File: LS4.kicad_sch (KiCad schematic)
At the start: 6 parts, among them U7 VNLD5160TR-E, U8 VNLD5160TR-E

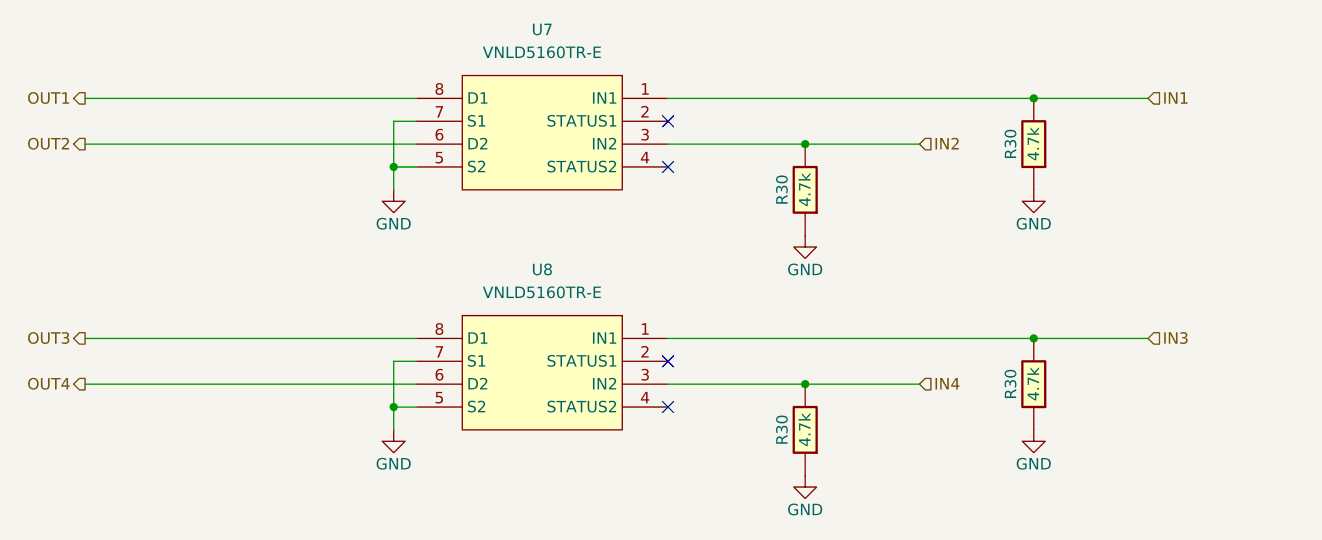
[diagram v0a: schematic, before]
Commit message: Unification with UAEFI F7 #114 #110
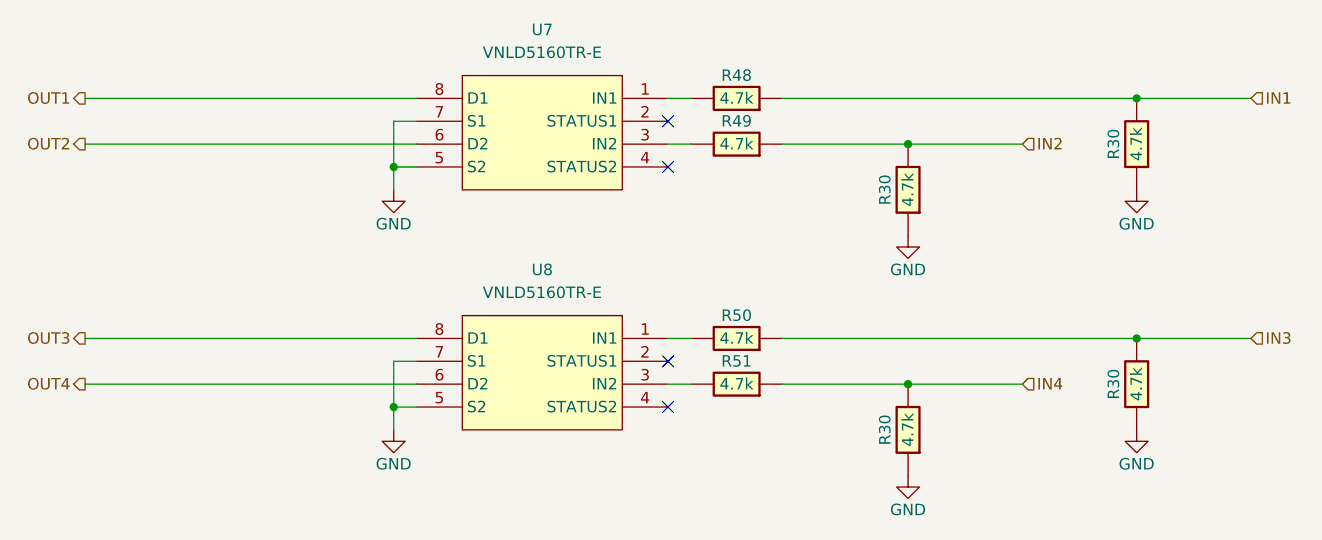
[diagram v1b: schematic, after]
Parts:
- added R48, R49, R50, R51: 4.7k, hellen-one-common:R0603, symbol hellen-one-common:Res
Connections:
- net IN1: now also R48.1; no longer U7.1 (IN1)
- net IN2: now also R49.1; no longer U7.3 (IN2)
- net IN3: now also R50.1; no longer U8.1 (IN1)
- net IN4: now also R51.1; no longer U8.3 (IN2)
- new net: R49.2, U7.3 (IN2)
- new net: R50.2, U8.1 (IN1)
- new net: R51.2, U8.3 (IN2)
- new net: R48.2, U7.1 (IN1)
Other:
- moved on the sheet: R30
